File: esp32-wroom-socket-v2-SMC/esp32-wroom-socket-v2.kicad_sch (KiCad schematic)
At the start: 9 parts, among them SW1 PRG, U1 ESP32-WROOM-32D

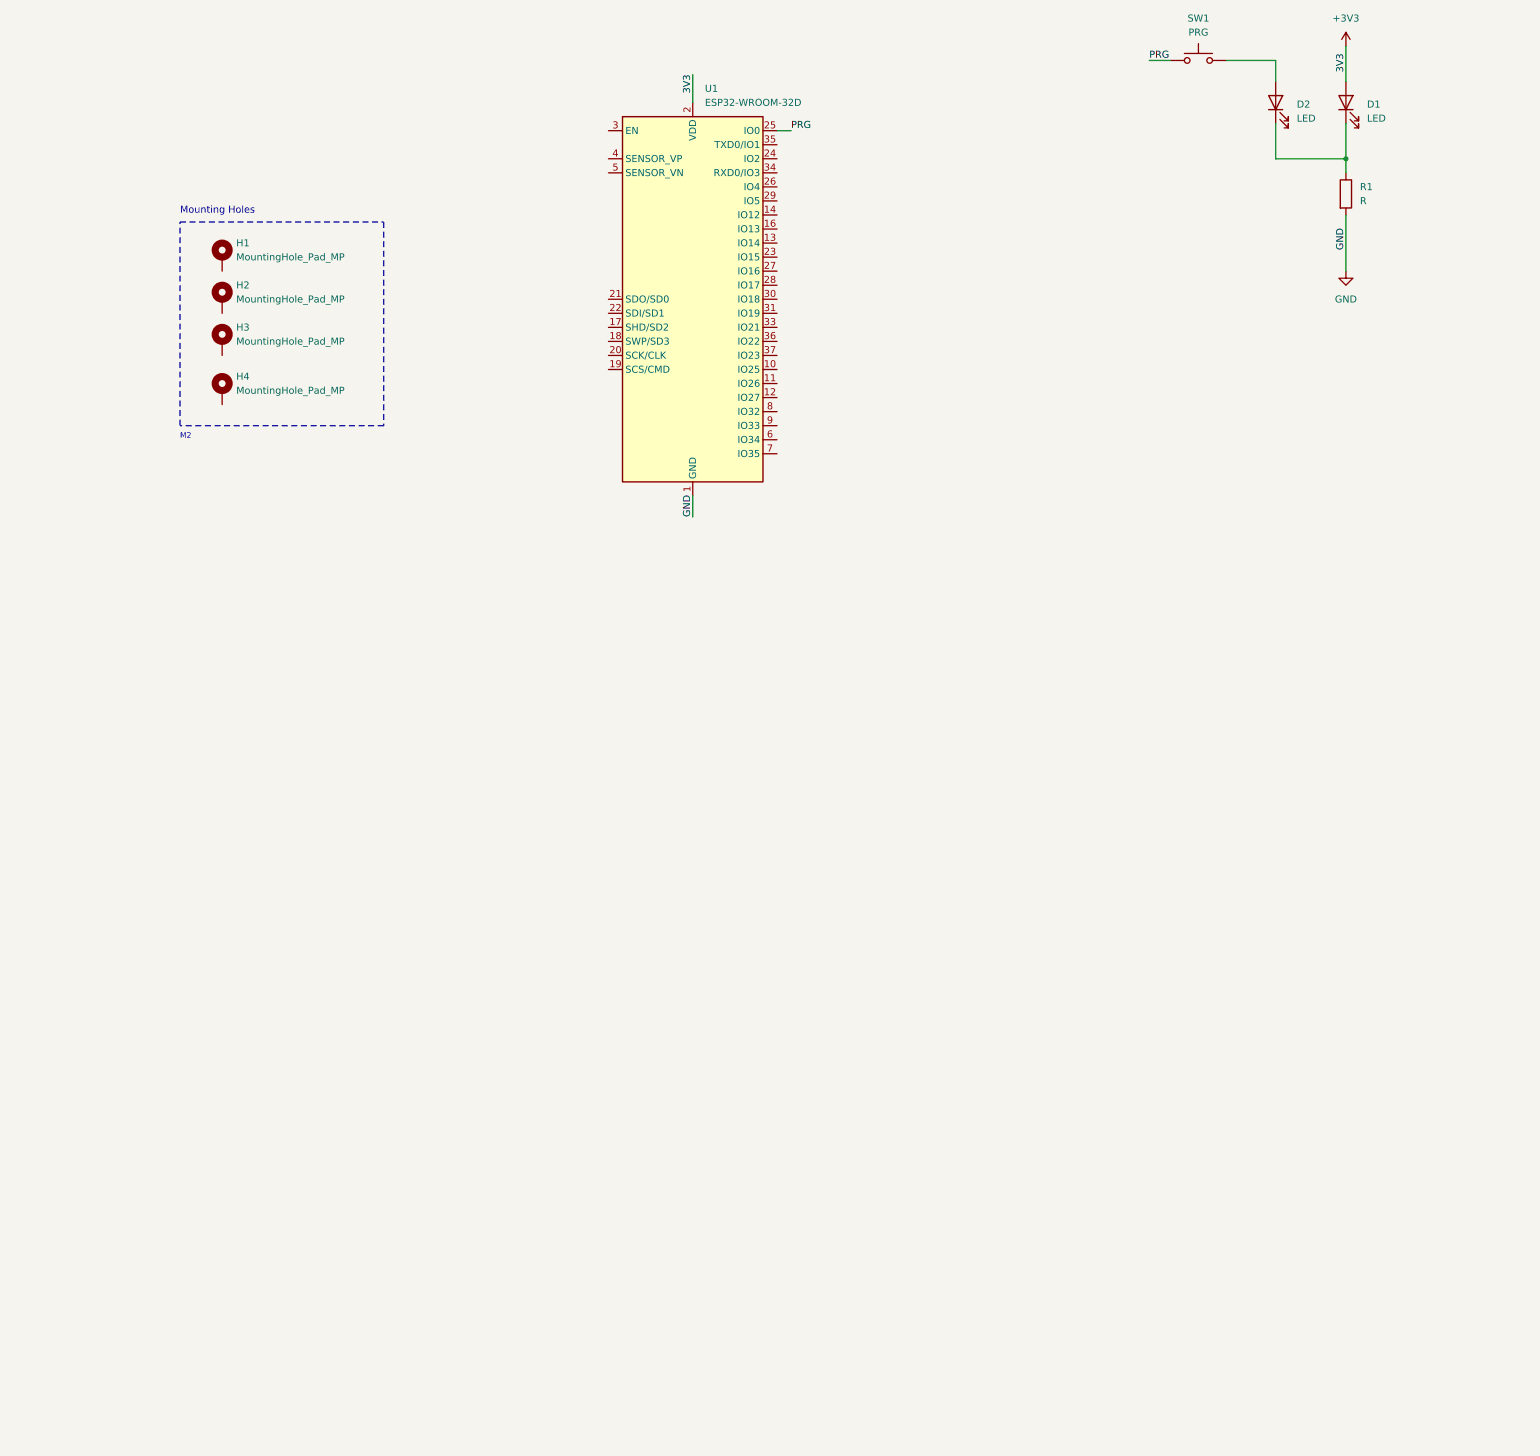
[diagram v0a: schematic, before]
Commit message: .
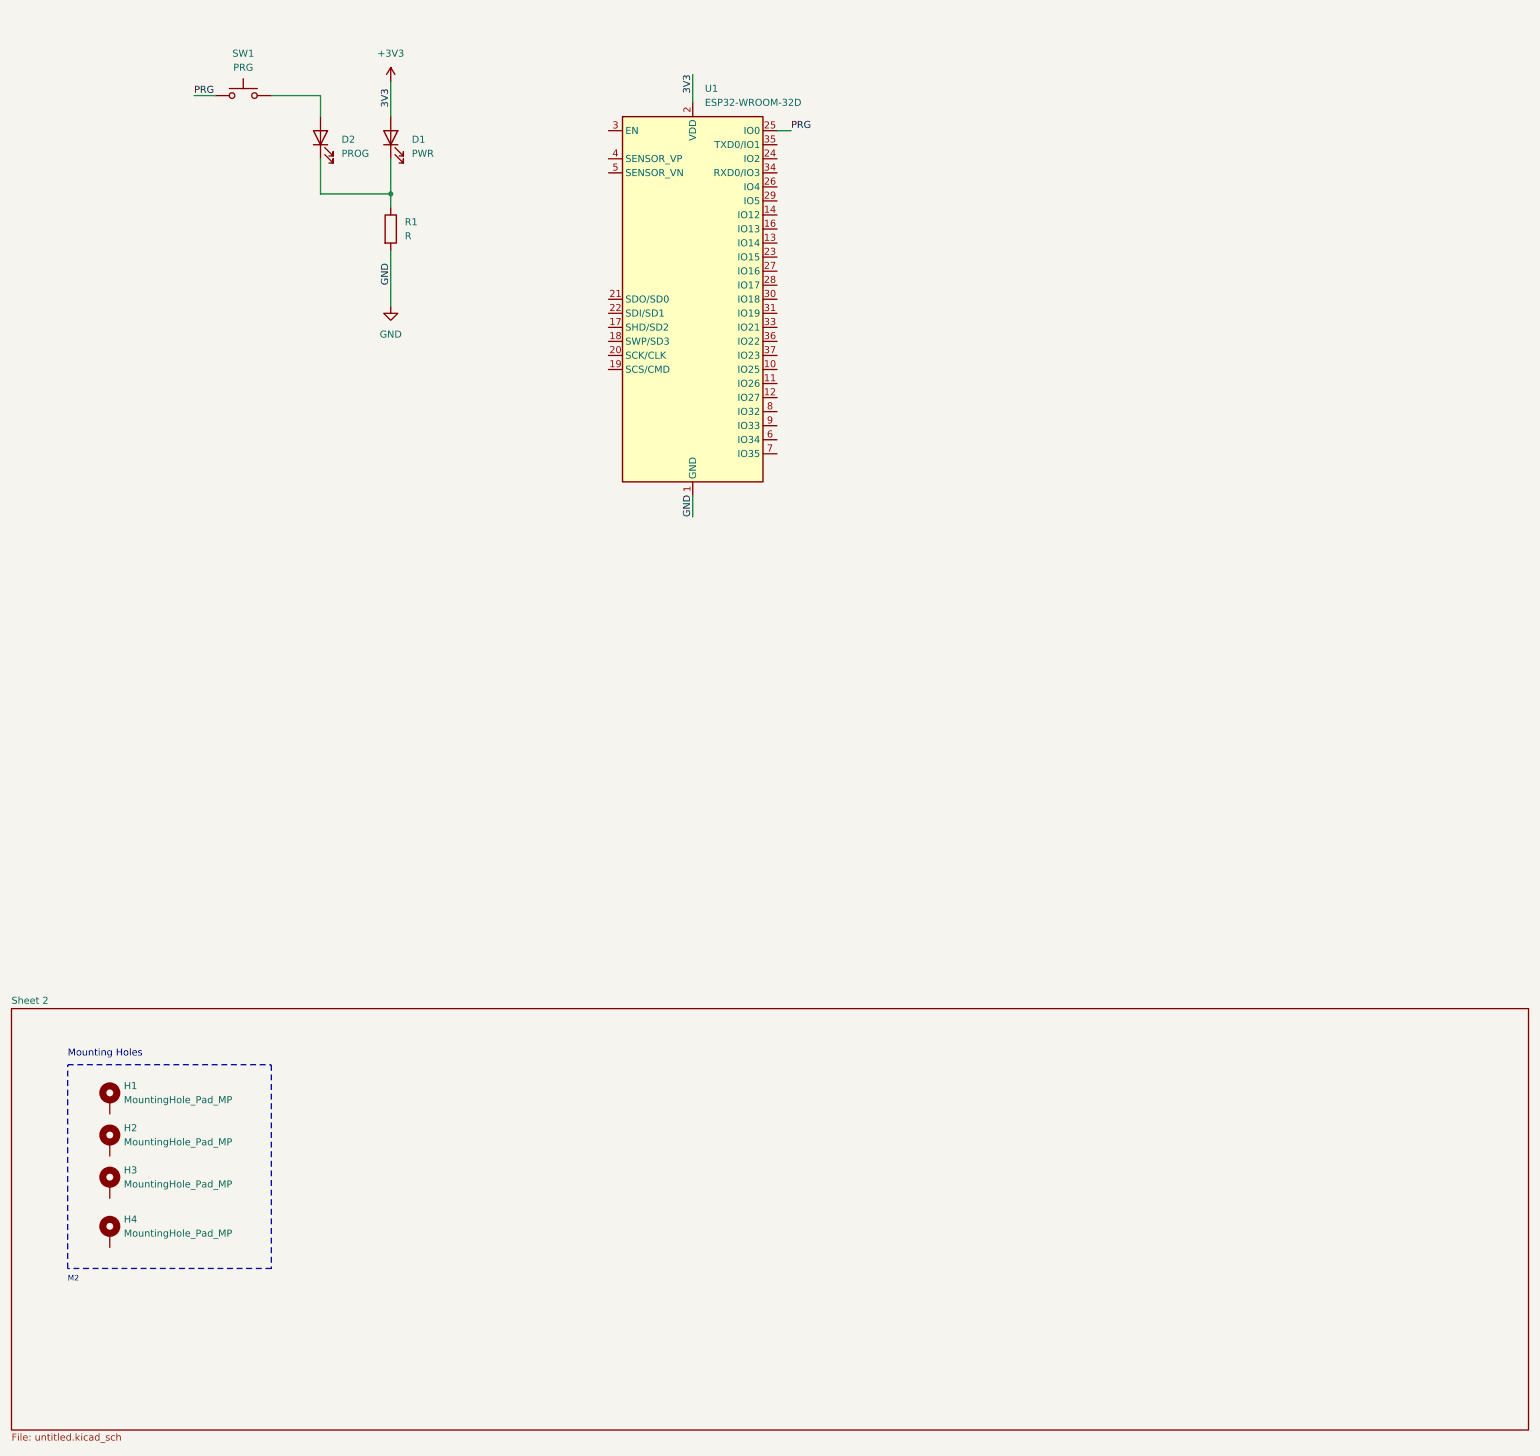
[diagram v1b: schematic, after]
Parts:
- D1: value LED -> PWR
- D2: value LED -> PROG
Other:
- added sheet Sheet 2 (untitled.kicad_sch)
- moved on the sheet: D1, D2, H1, H2, H3, H4, R1, SW1
